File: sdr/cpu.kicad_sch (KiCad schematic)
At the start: 30 parts, among them J2 Conn_01x06, SW1 RESET, SW2 KEY, SW3 PTT, U4 CH32V305RBT6, Y2 25MHz

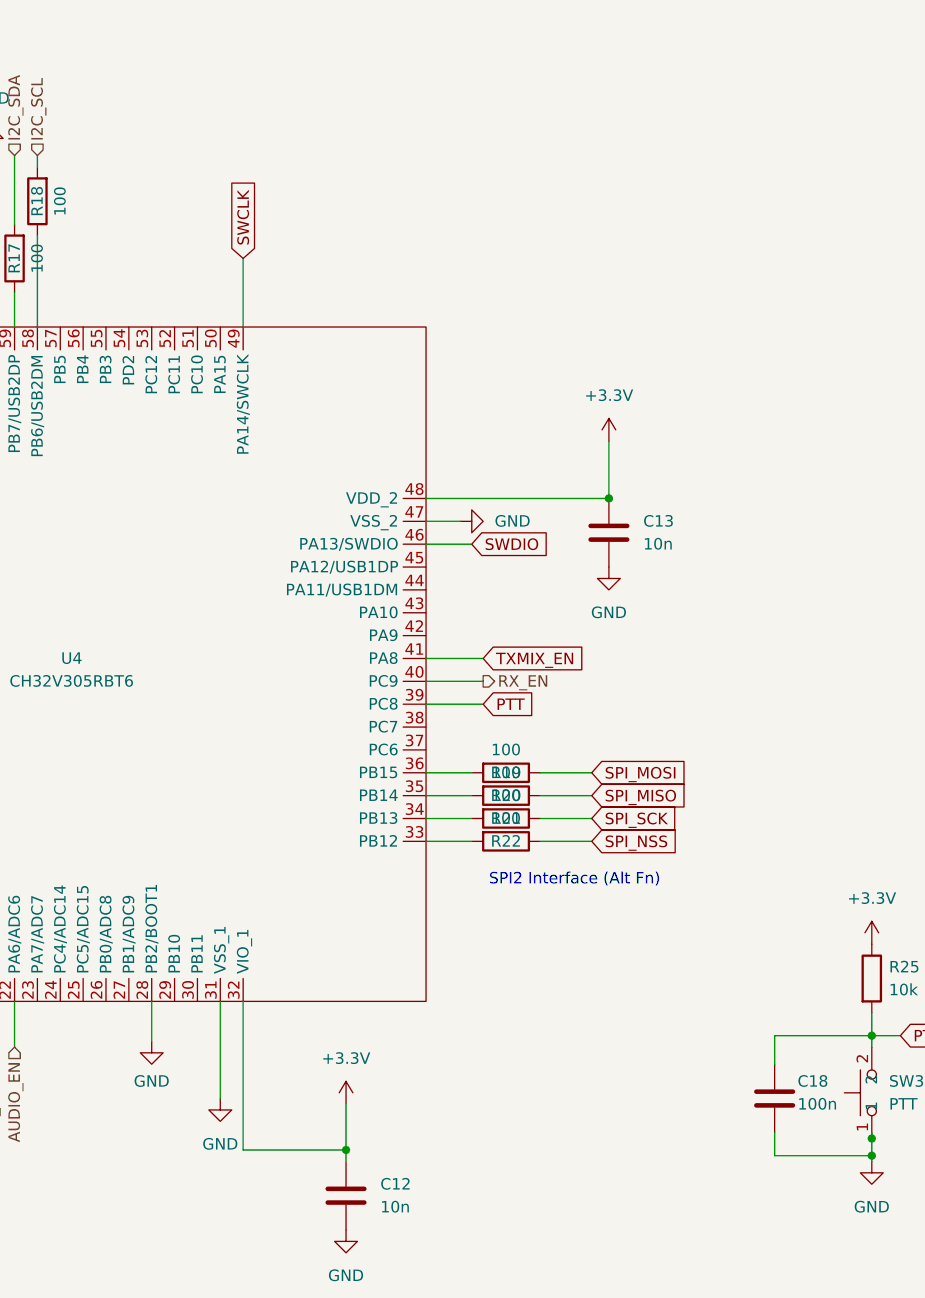
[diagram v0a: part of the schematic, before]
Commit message: First version 0.1 completed
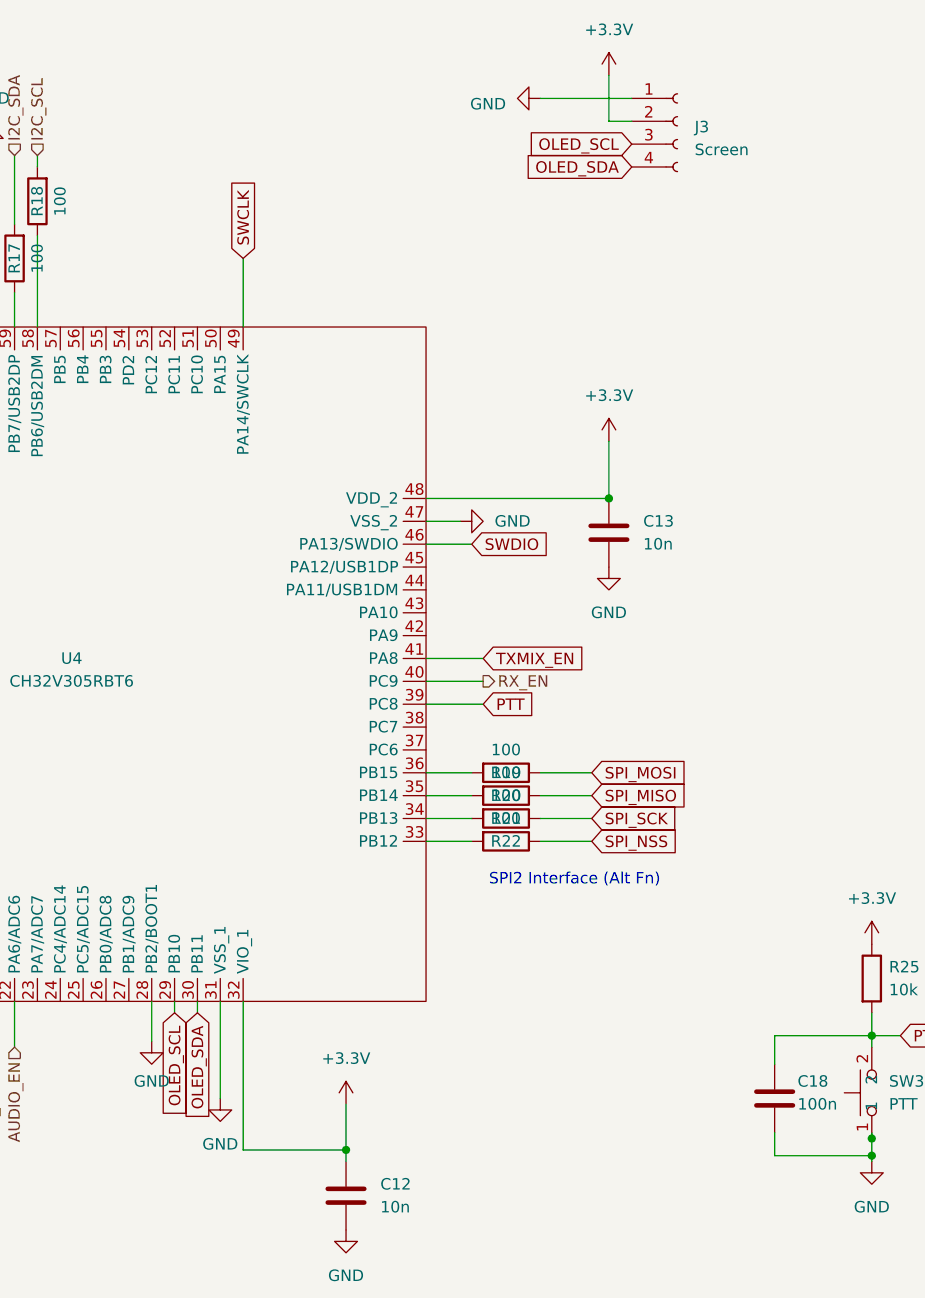
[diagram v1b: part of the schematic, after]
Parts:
- added J3: Screen, Connector_PinSocket_2.54mm:PinSocket_1x04_P2.54mm_Vertical, symbol Connector:Conn_01x04_Socket
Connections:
- net +3.3V: now also J3.2 (Pin_2)
- net GND: now also J3.1 (Pin_1)
- net OLED_SCL: now reaches U4.29 (PB10)
- net OLED_SCL: now also J3.3 (Pin_3)
- net OLED_SDA: now reaches U4.30 (PB11)
- net OLED_SDA: now also J3.4 (Pin_4)
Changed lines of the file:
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@@
+    (stroke (width 0) (type default))
+  )
+  (wire (pts (xy 176.53 41.91) (xy 173.99 41.91))
     (stroke (width 0) (type default))
   )
@@
     (stroke (width 0) (type default))
   )
+  (wire (pts (xy 166.37 39.37) (xy 176.53 39.37))
+    (stroke (width 0) (type default))
+  )
   (wire (pts (xy 107.95 60.96) (xy 107.95 64.77))
     (stroke (width 0) (type default))
@@
     (stroke (width 0) (type default))
   )
+  (wire (pts (xy 128.27 139.7) (xy 128.27 140.97))
+    (stroke (width 0) (type default))
+  )
   (wire (pts (xy 192.405 154.305) (xy 192.405 156.845))
     (stroke (width 0) (type default))
@@
     (stroke (width 0) (type default))
   )
+  (wire (pts (xy 125.73 139.7) (xy 125.73 140.97))
+    (stroke (width 0) (type default))
+  )
   (wire (pts (xy 76.2 96.52) (xy 54.61 96.52))
     (stroke (width 0) (type default))
@@
   )
   (wire (pts (xy 97.79 52.07) (xy 92.075 52.07))
+    (stroke (width 0) (type default))
+  )
+  (wire (pts (xy 173.99 41.91) (xy 173.99 36.83))
     (stroke (width 0) (type default))
   )
@@
     (effects (font (size 1.27 1.27)) (justify left bottom))
   )
+  (global_label "OLED_SDA" (shape input) (at 176.53 46.99 180) (fields_autoplaced)
+    (effects (font (size 1.27 1.27)) (justify right))
+    (property "Intersheetrefs" "${INTERSHEET_REFS}" (at 164.3109 46.99 0)
+      (effects (font (size 1.27 1.27)) (justify right) hide)
+    )
+  )
   (global_label "NRST" (shape input) (at 226.06 76.2 180) (fields_autoplaced)
     (effects (font (size 1.27 1.27)) (justify right))
@@
     )
   )
+  (global_label "OLED_SDA" (shape input) (at 128.27 140.97 270) (fields_autoplaced)
+    (effects (font (size 1.27 1.27)) (justify right))
+    (property "Intersheetrefs" "${INTERSHEET_REFS}" (at 128.27 153.1891 90)
+      (effects (font (size 1.27 1.27)) (justify right) hide)
+    )
+  )
   (global_label "SWCLK" (shape input) (at 133.35 57.15 90) (fields_autoplaced)
     (effects (font (size 1.27 1.27)) (justify left))
@@
     )
   )
+  (global_label "OLED_SCL" (shape input) (at 125.73 140.97 270) (fields_autoplaced)
+    (effects (font (size 1.27 1.27)) (justify right))
+    (property "Intersheetrefs" "${INTERSHEET_REFS}" (at 125.73 153.1286 90)
+      (effects (font (size 1.27 1.27)) (justify right) hide)
+    )
+  )
   (global_label "SPI_MISO" (shape input) (at 172.085 116.84 0) (fields_autoplaced)
     (effects (font (size 1.27 1.27)) (justify left))
@@
     (property "Intersheetrefs" "${INTERSHEET_REFS}" (at 167.0293 88.8206 0)
       (effects (font (size 1.27 1.27)) (justify left) hide)
+    )
+  )
+  (global_label "OLED_SCL" (shape input) (at 176.53 44.45 180) (fields_autoplaced)
+    (effects (font (size 1.27 1.27)) (justify right))
+    (property "Intersheetrefs" "${INTERSHEET_REFS}" (at 164.3714 44.45 0)
+      (effects (font (size 1.27 1.27)) (justify right) hide)
     )
   )
@@
     )
   )
+  (symbol (lib_id "Connector:Conn_01x04_Socket") (at 181.61 41.91 0) (unit 1)
+    (in_bom yes) (on_board yes) (dnp no) (fields_autoplaced)
+    (property "Reference" "J3" (at 183.515 42.545 0)
+      (effects (font (size 1.27 1.27)) (justify left))
+    )
+    (property "Value" "Screen" (at 183.515 45.085 0)
+      (effects (font (size 1.27 1.27)) (justify left))
+    )
+    (property "Footprint" "Connector_PinSocket_2.54mm:PinSocket_1x04_P2.54mm_Vertical" (at 181.61 41.91 0)
+      (effects (font (size 1.27 1.27)) hide)
+    )
+    (property "Datasheet" "~" (at 181.61 41.91 0)
+      (effects (font (size 1.27 1.27)) hide)
+    )
+    (pin "1")
+    (pin "2")
+    (pin "3")
+    (pin "4")
+    (instances
+      (project "attorv"
+        (path "/6109b252-c3cf-4e79-aa0f-a13bf7f36f08"
+          (reference "J3") (unit 1)
+        )
+      )
+      (project "sdr"
+        (path "/ee974380-b45b-4b16-8475-50e4e51dc6cf/ad7b2242-3b39-40b3-b2e9-d6ea800dea9e"
+          (reference "J5") (unit 1)
+        )
+      )
+    )
+  )
   (symbol (lib_id "power:GND") (at 41.91 124.46 0) (unit 1)
     (in_bom yes) (on_board yes) (dnp no) (fields_autoplaced)
@@
     )
   )
+  (symbol (lib_id "power:GND") (at 166.37 39.37 270) (unit 1)
+    (in_bom yes) (on_board yes) (dnp no) (fields_autoplaced)
+    (property "Reference" "#PWR017" (at 160.02 39.37 0)
+      (effects (font (size 1.27 1.27)) hide)
+    )
+    (property "Value" "GND" (at 162.56 40.005 90)
+      (effects (font (size 1.27 1.27)) (justify right))
+    )
+    (property "Footprint" "" (at 166.37 39.37 0)
+      (effects (font (size 1.27 1.27)) hide)
+    )
+    (property "Datasheet" "" (at 166.37 39.37 0)
+      (effects (font (size 1.27 1.27)) hide)
+    )
+    (property "JLCPCB" "C2296" (at 166.37 39.37 0)
+      (effects (font (size 1.27 1.27)) hide)
+    )
+    (pin "1")
+    (instances
+      (project "attorv"
+        (path "/6109b252-c3cf-4e79-aa0f-a13bf7f36f08"
+          (reference "#PWR017") (unit 1)
+        )
+      )
+      (project "batomatic"
+        (path "/6a22bd48-0d2f-47d1-9720-f349a7ed8e38"
+          (reference "#PWR0102") (unit 1)
+        )
+      )
+      (project "sdr"
+        (path "/ee974380-b45b-4b16-8475-50e4e51dc6cf/ad7b2242-3b39-40b3-b2e9-d6ea800dea9e"
+          (reference "#PWR056") (unit 1)
+        )
+      )
+    )
+  )
   (symbol (lib_id "power:GND") (at 85.09 168.91 0) (unit 1)
     (in_bom yes) (on_board yes) (dnp no) (fields_autoplaced)
@@
         )
       )
+    )
+  )
+  (symbol (lib_id "power:+3.3V") (at 173.99 36.83 0) (unit 1)
+    (in_bom yes) (on_board yes) (dnp no) (fields_autoplaced)
+    (property "Reference" "#PWR018" (at 173.99 40.64 0)
+      (effects (font (size 1.27 1.27)) hide)
+    )
+    (property "Value" "+3.3V" (at 173.99 31.75 0)
+      (effects (font (size 1.27 1.27)))
+    )
+    (property "Footprint" "" (at 173.99 36.83 0)
+      (effects (font (size 1.27 1.27)) hide)
+    )
+    (property "Datasheet" "" (at 173.99 36.83 0)
+      (effects (font (size 1.27 1.27)) hide)
+    )
+    (pin "1")
+    (instances
+      (project "attorv"
+        (path "/6109b252-c3cf-4e79-aa0f-a13bf7f36f08"
+          (reference "#PWR018") (unit 1)
+        )
+      )
+      (project "batomatic"
+        (path "/6a22bd48-0d2f-47d1-9720-f349a7ed8e38"
+          (reference "#PWR017") (unit 1)
+        )
+      )
+      (project "sdr"
+        (path "/ee974380-b45b-4b16-8475-50e4e51dc6cf/ad7b2242-3b39-40b3-b2e9-d6ea800dea9e"
+          (reference "#PWR059") (unit 1)
+        )
+      )
